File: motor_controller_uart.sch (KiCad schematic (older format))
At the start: 38 parts, among them J10 DB9_Male, J11 DB9_Male, J8 DB9_Male, J9 DB9_Male, U2 MAX3232, U4 MAX3232

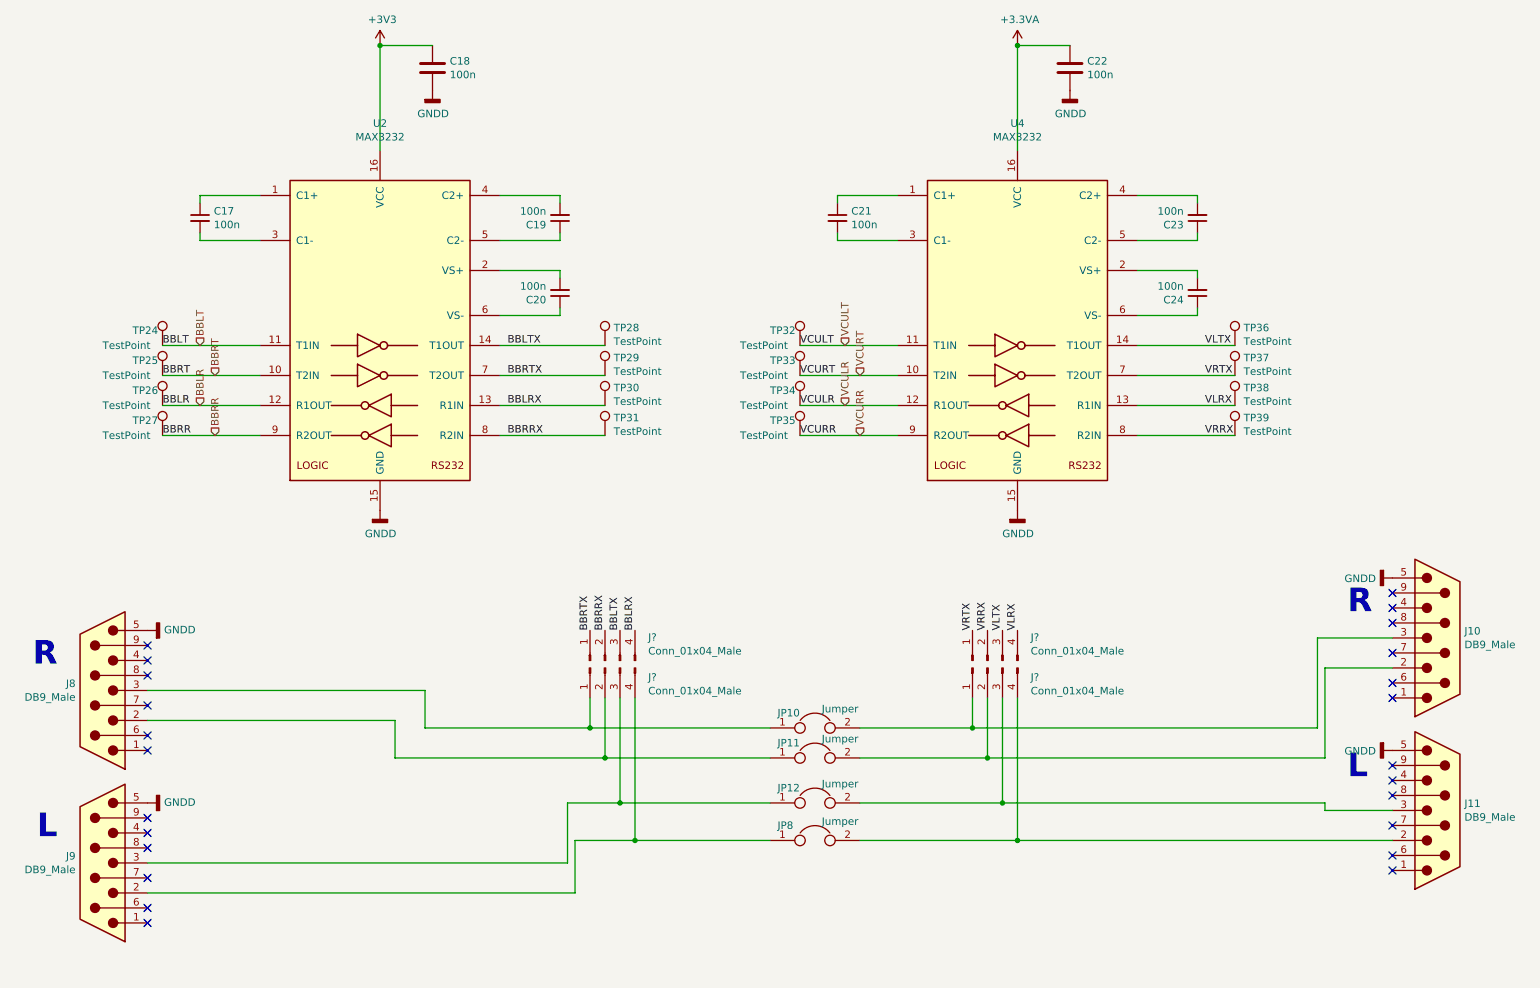
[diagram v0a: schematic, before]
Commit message: rs232 fix
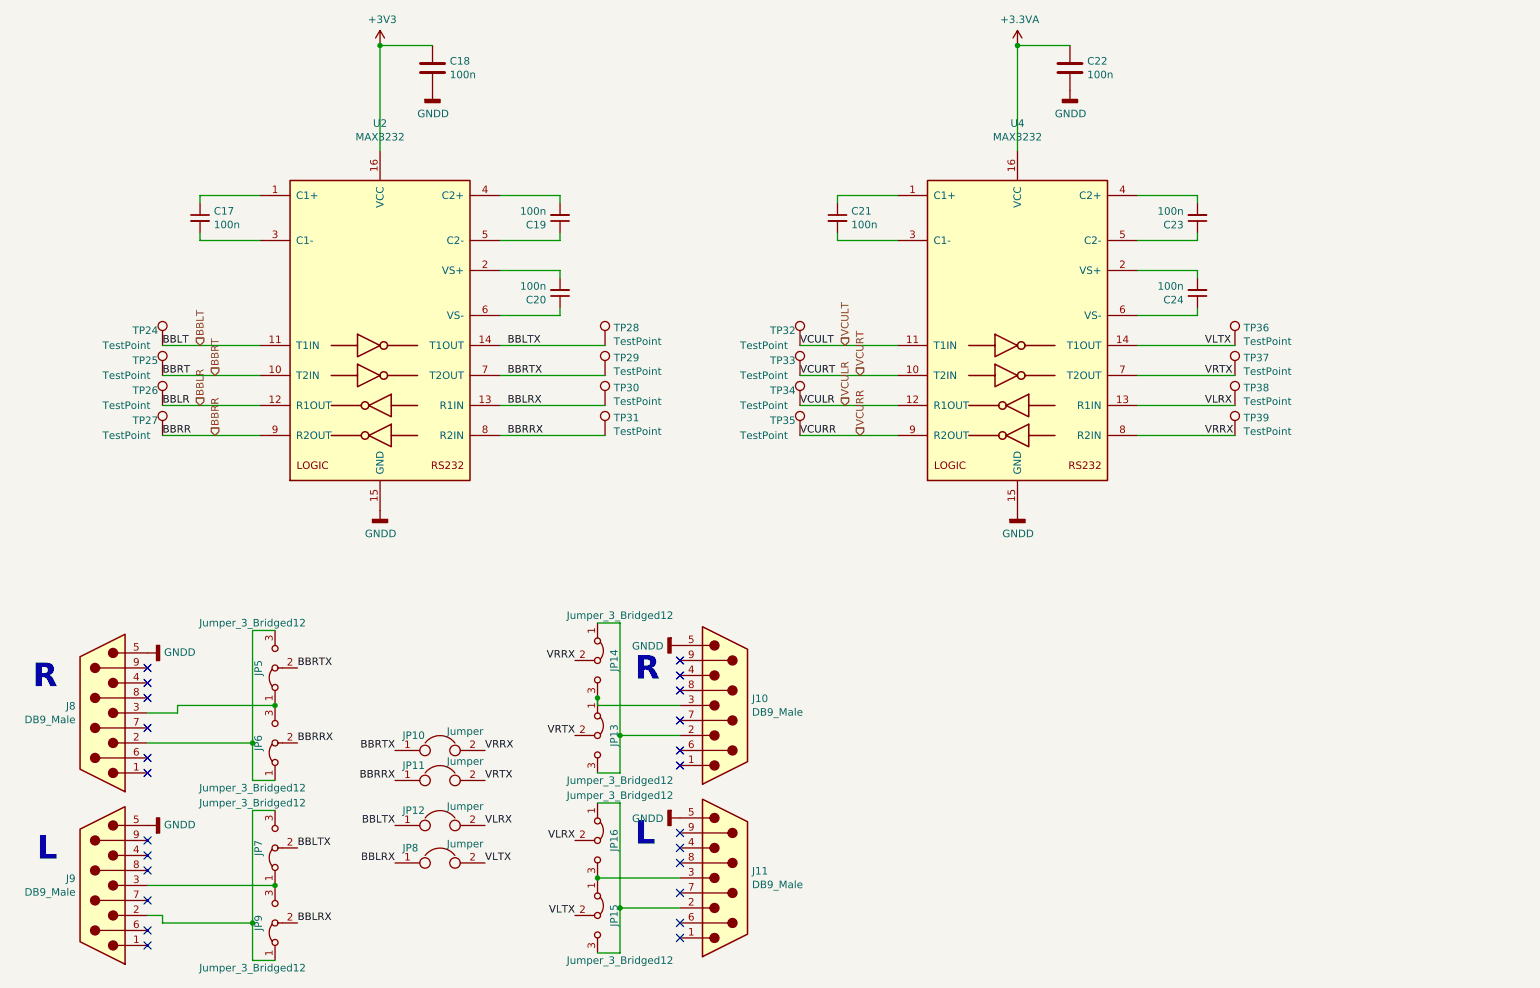
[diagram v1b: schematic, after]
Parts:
- removed J? (x4): Conn_01x04_Male, symbol Connector:Conn_01x04_Male
- added JP13, JP14, JP15, JP16, JP5, JP6, JP7, JP9: Jumper_3_Bridged12, Connector_PinHeader_2.00mm:PinHeader_1x03_P2.00mm_Vertical, symbol Jumper:Jumper_3_Bridged12
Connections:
- net BBLRX: now also JP8.1, JP9.2 (C)
- net BBLTX: now also JP12.1, JP7.2 (C)
- net BBRRX: now also JP11.1, JP6.2 (C)
- net BBRTX: now also JP10.1, JP5.2 (C)
- net VLRX: now also JP12.2, JP16.2 (C)
- net VLTX: now also JP8.2, JP15.2 (C)
- net VRRX: now also JP10.2, JP14.2 (C)
- net VRTX: now also JP11.2, JP13.2 (C)
- net at J9.3: now also JP7.1 (A), JP9.3 (B); no longer JP12.1
- net at J11.3: now also JP15.1 (A), JP16.3 (B); no longer JP12.2
- net at J8.2: now also JP5.3 (B), JP6.1 (A); no longer JP11.1
- net at J10.2: now also JP13.3 (B), JP14.1 (A); no longer JP11.2
- net at J8.3: now also JP5.1 (A), JP6.3 (B); no longer JP10.1
- net at J10.3: now also JP13.1 (A), JP14.3 (B); no longer JP10.2
- net at J9.2: now also JP7.3 (B), JP9.1 (A); no longer JP8.1
- net at J11.2: now also JP15.3 (B), JP16.1 (A); no longer JP8.2
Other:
- moved on the sheet: J10, J11, J8, J9, JP10, JP11, JP12, JP8
